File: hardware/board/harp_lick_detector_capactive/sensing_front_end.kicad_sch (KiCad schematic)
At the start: 29 parts

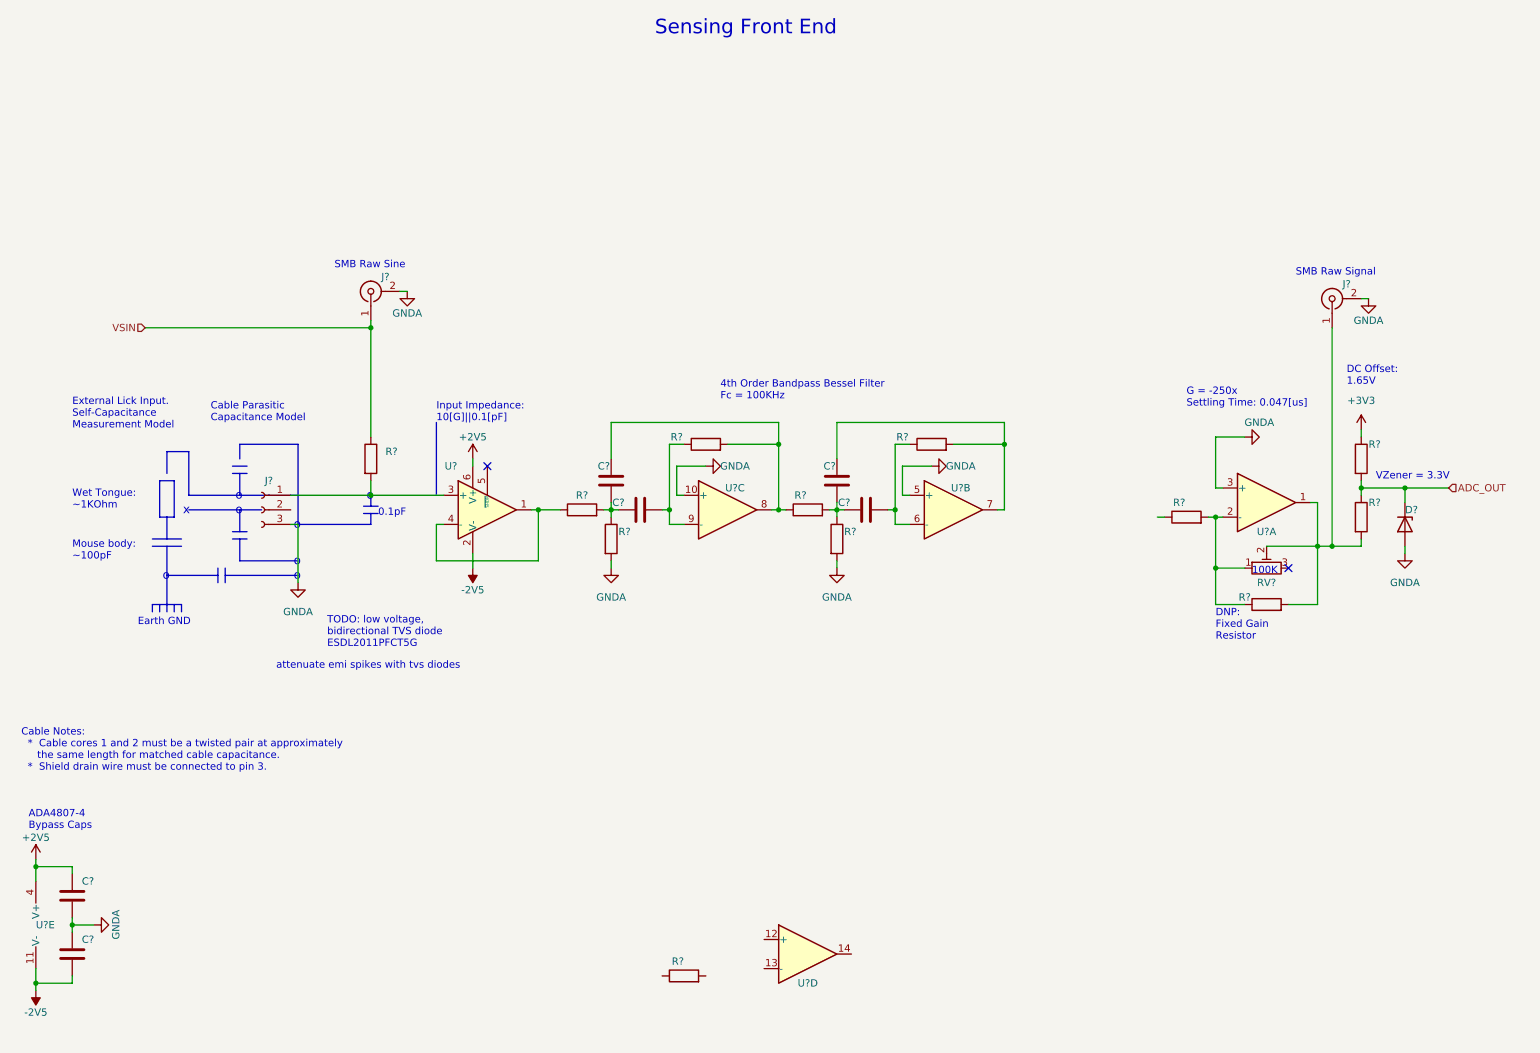
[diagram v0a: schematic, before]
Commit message: add driven shield
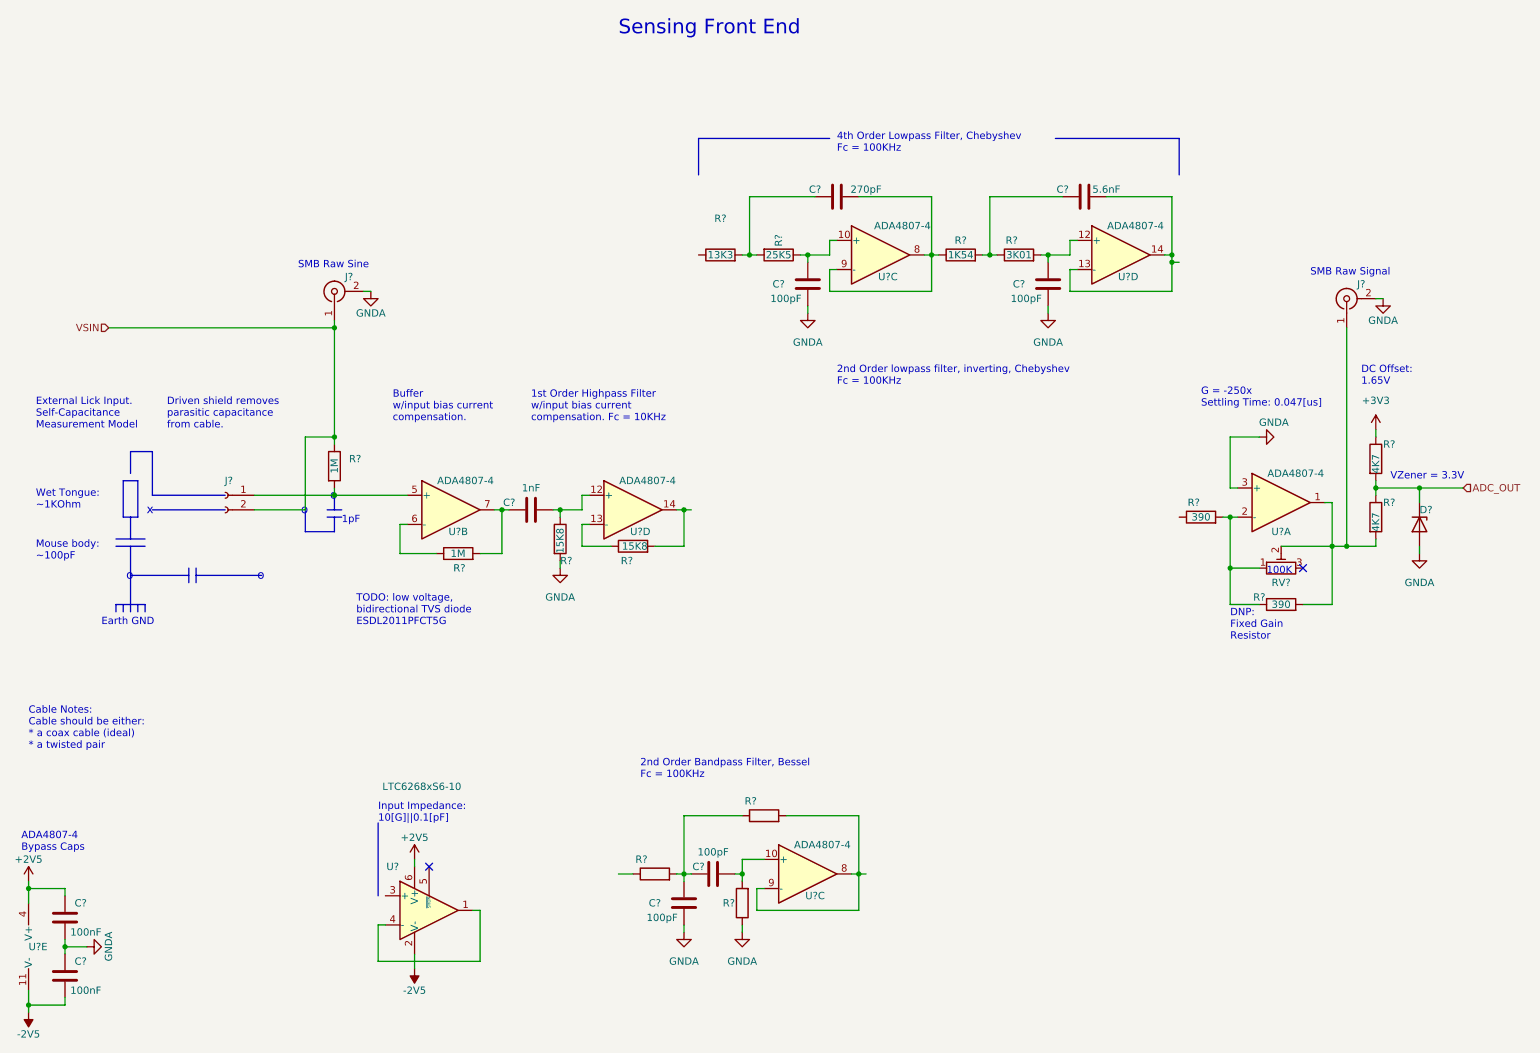
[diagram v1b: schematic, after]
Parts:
- removed C? (x3): (no value), symbol Device:C
- removed J?: (no value), symbol Connector:Conn_01x03_Female
- removed R? (x7): (no value), symbol Device:R
- added C? (x3): 100pF, Capacitor_SMD:C_0603_1608Metric_Pad1.08x0.95mm_HandSolder, symbol Device:C
- added C?: 1nF, symbol Device:C
- added C?: 5.6nF, symbol Device:C
- added C?: 270pF, symbol Device:C
- added J?: (no value), symbol Connector:Conn_01x02_Female
- added R? (x3): (no value), symbol Device:R
- added R?: 13K3, symbol Device:R
- added R? (x2): 15K8, symbol Device:R
- added R?: 25K5, symbol Device:R
- added R?: 1M, Resistor_SMD:R_0603_1608Metric_Pad0.98x0.95mm_HandSolder, symbol Device:R
- added R?: 1K54, symbol Device:R
- added R?: 3K01, symbol Device:R
- added U? (x2): ADA4807-4, Package_SO:TSSOP-14_4.4x5mm_P0.65mm, symbol Amplifier_Operational:ADA4807-4
- C? (x2): value (none) -> 100nF; footprint (none) -> Capacitor_SMD:C_0603_1608Metric_Pad1.08x0.95mm_HandSolder
- C?: value (none) -> 100pF; footprint (none) -> Capacitor_SMD:C_0603_1608Metric_Pad1.08x0.95mm_HandSolder
- D?: value (none) -> BZX384-A3V3-QX; footprint (none) -> Diode_SMD:D_SOD-323_HandSoldering
- J? (x2): value (none) -> Conn_Coaxial; footprint (none) -> Connector_Coaxial:SMA_Amphenol_901-143_Horizontal
- R?: value (none) -> 1M; footprint (none) -> Resistor_SMD:R_0603_1608Metric_Pad0.98x0.95mm_HandSolder
- R? (x2): value (none) -> 4K7; footprint (none) -> Resistor_SMD:R_0603_1608Metric_Pad0.98x0.95mm_HandSolder
- R? (x2): value (none) -> 390; footprint (none) -> Resistor_SMD:R_0603_1608Metric_Pad0.98x0.95mm_HandSolder
- RV?: value (none) -> R_Potentiometer_Trim; footprint (none) -> Potentiometer_SMD:Potentiometer_Bourns_3314G_Vertical
- U? (x5): value (none) -> ADA4807-4; footprint (none) -> Package_SO:TSSOP-14_4.4x5mm_P0.65mm
- U?: value (none) -> LTC6268xS6-10
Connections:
- net GNDA: now also C?.1, C?.1, C?.1, R?.1, R?.2; no longer U?.10 (+), U?.5 (+)
- net VSIN: now also J?.2 (Pin_2)
- net at U?.6 (-): now also R?.1
- net at U?.3 (+): no longer R?.2
- net at U?.8: now also U?.9 (-), C?.2, R?.1
- net at C?.2: now also U?.10 (+), R?.1; no longer U?.7
- net at U?.12 (+): now also C?.2, R?.1
- net at U?.13 (-): now also R?.1
- net at U?.14: now also R?.2
- new net: C?.2, R?.2, U?.12 (+)
- new net: C?.2, U?.13 (-), U?.14
- new net: C?.1, R?.2, U?.10 (+)
- new net: C?.1, R?.2, R?.2
- new net: C?.2, C?.2, R?.1, R?.2
- new net: J?.1 (Pin_1), R?.2, U?.5 (+)
- new net: C?.1, R?.2, U?.7
- new net: C?.1, R?.1, R?.2
- new net: R?.2, U?.8, U?.9 (-)
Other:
- note added: "1pF"
- note added: "1st Order Highpass Filter w/input bias current compensation. Fc = 10KHz"
- note added: "2nd Order Bandpass Filter, Bessel Fc = 100KHz"
- note added: "2nd Order lowpass filter, inverting, Chebyshev Fc = 100KHz"
- note added: "4th Order Lowpass Filter, Chebyshev Fc = 100KHz"
- note added: "Buffer w/input bias current compensation."
- note added: "Cable Notes: Cable should be either: * a coax cable (ideal) * a twisted pair"
- note added: "Driven shield removes parasitic capacitance from cable."
- note removed: "0.1pF"
- note removed: "4th Order Bandpass Bessel Filter Fc = 100KHz"
- note removed: "Cable Notes: * Cable cores 1 and 2 must be a twisted pair at approximately the same length for matched cable capacitance. * Shield drain wire must be connected to pin 3."
- note removed: "Cable Parasitic Capacitance Model"
- note removed: "attenuate emi spikes with tvs diodes"
- moved on the sheet: C?, D?, J?, R?, RV?, U?, U?A, U?B, U?C, U?D, U?E
